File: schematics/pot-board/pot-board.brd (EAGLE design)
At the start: 97.8 x 30.2 mm, 16 parts, among them J3 POWER_JACKPTH_LOCK

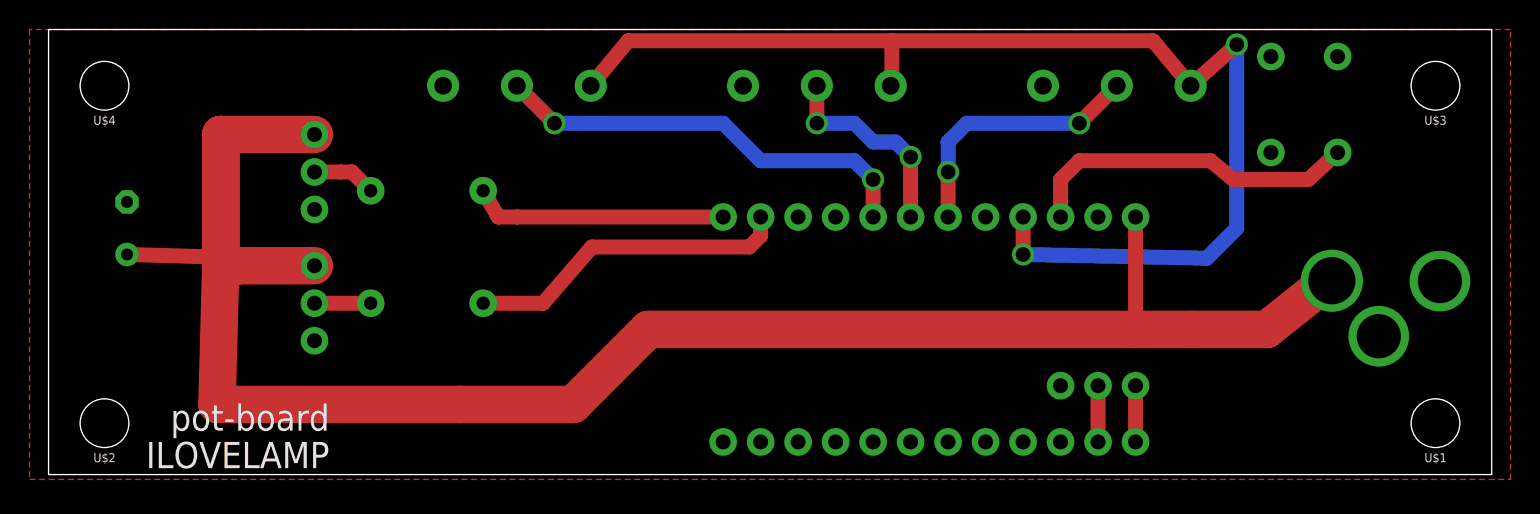
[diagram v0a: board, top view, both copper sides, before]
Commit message: small fixes
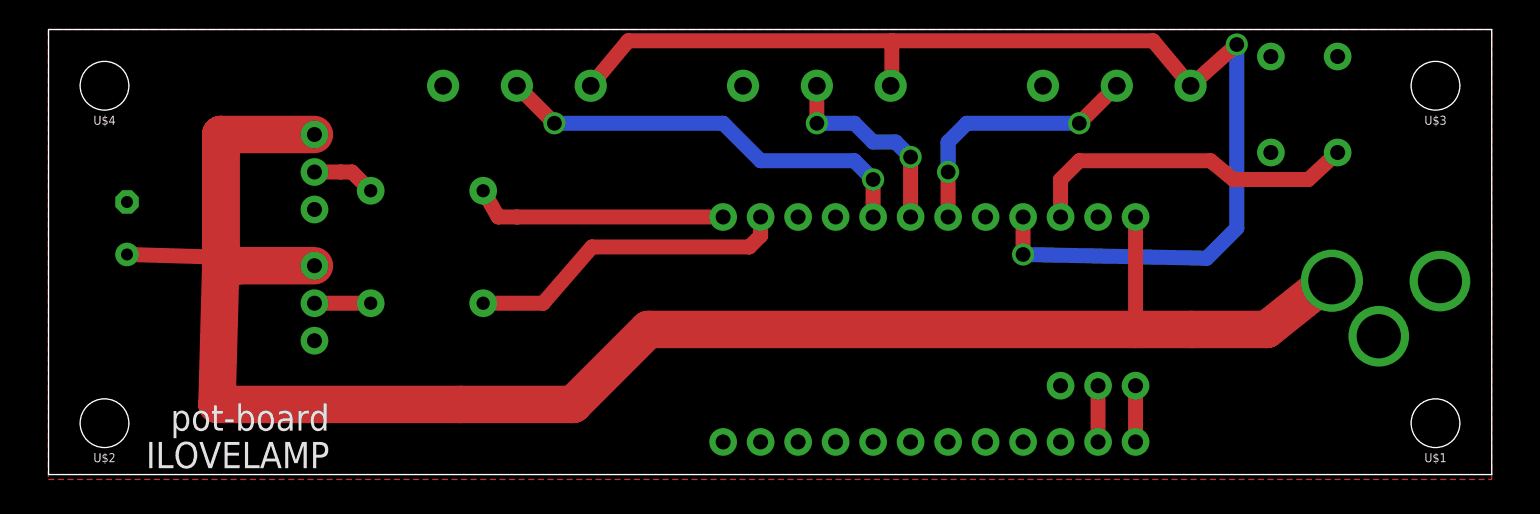
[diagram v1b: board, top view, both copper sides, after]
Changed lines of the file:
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@@
 <contactref element="J2" pad="3"/>
 <polygon width="1.016" layer="1">
-<vertex x="-1.27" y="0"/>
-<vertex x="99.06" y="0"/>
-<vertex x="99.06" y="30.48"/>
-<vertex x="-1.27" y="30.48"/>
+<vertex x="0" y="0"/>
+<vertex x="97.79" y="0"/>
+<vertex x="97.79" y="30.48"/>
+<vertex x="0" y="30.48"/>
 </polygon>
 <contactref element="S4" pad="3"/>
